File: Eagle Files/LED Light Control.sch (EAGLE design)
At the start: 9 parts, among them IC1 LM317MBSTT3

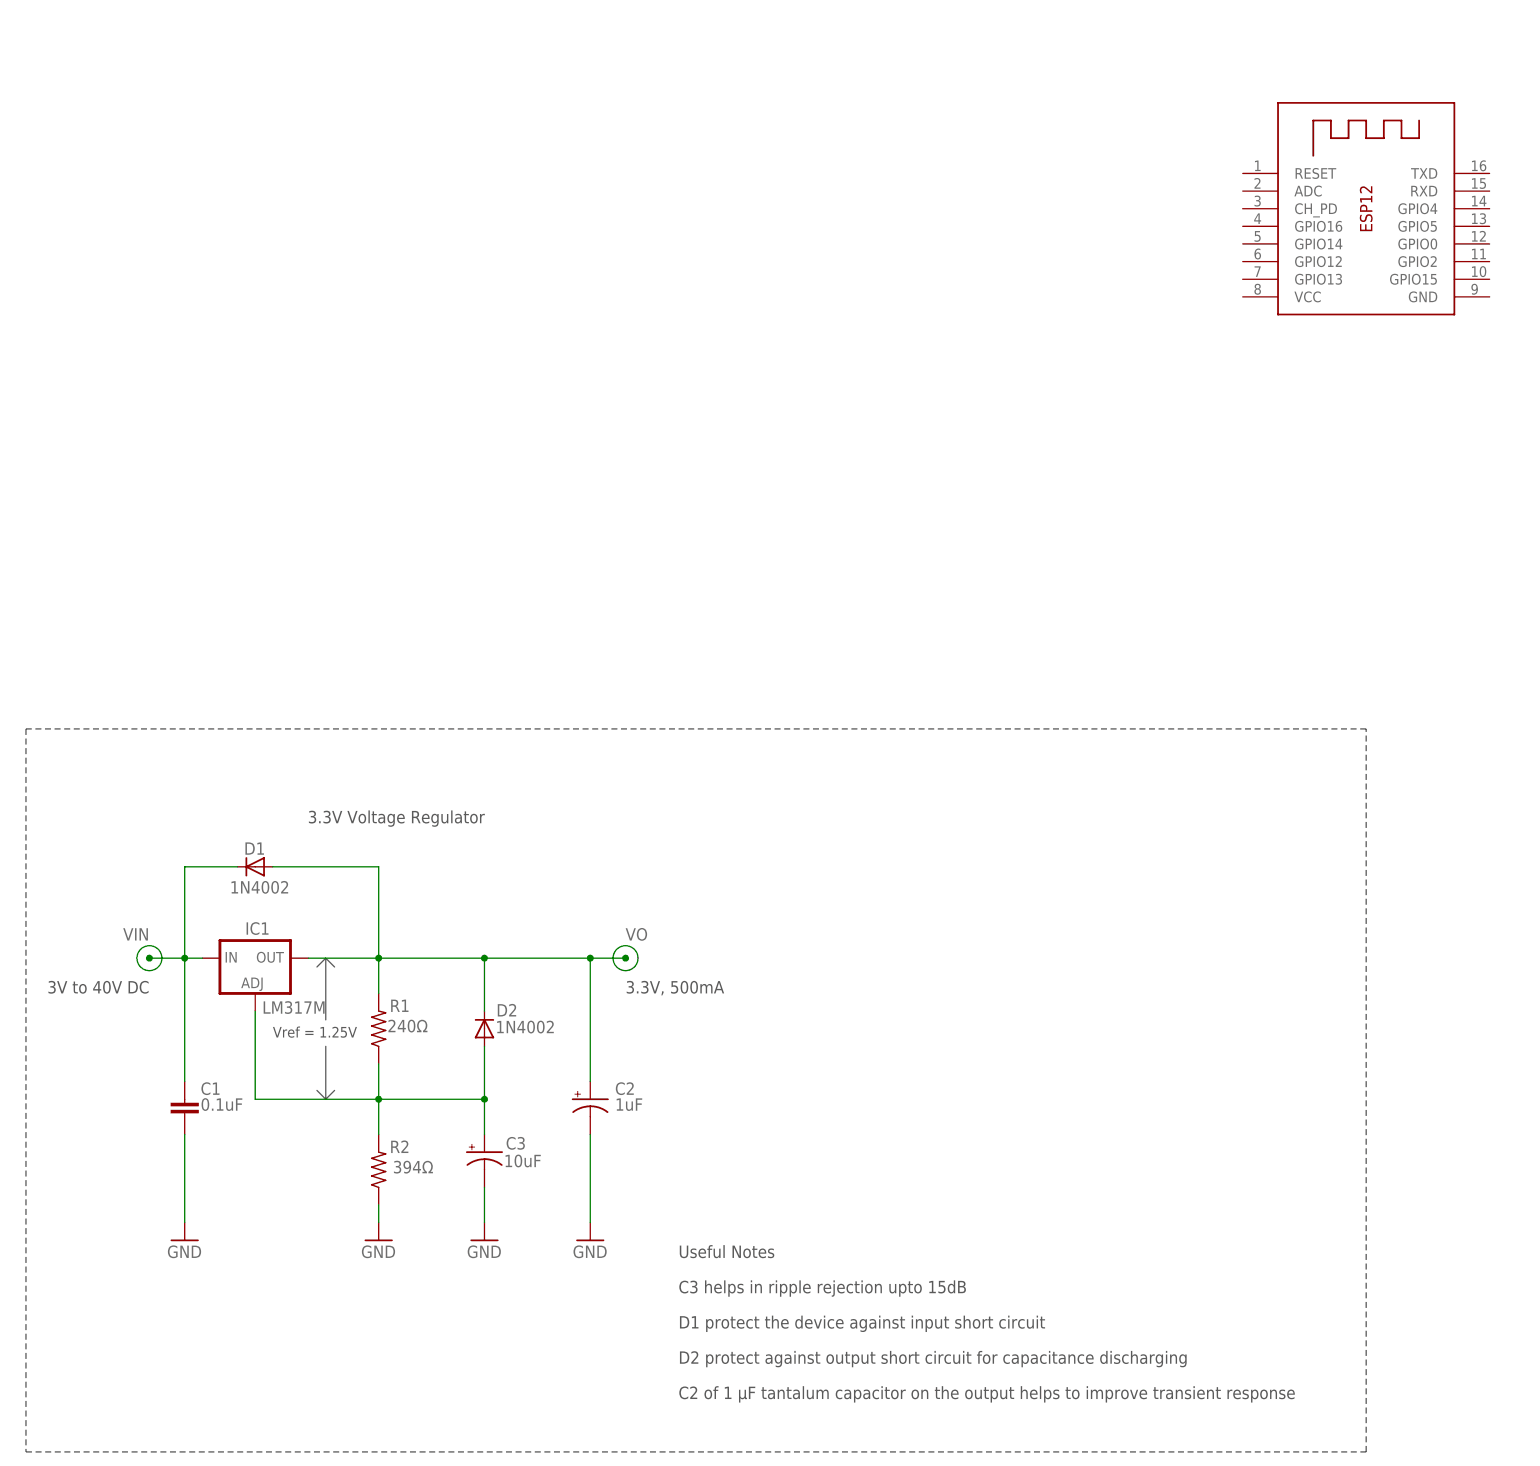
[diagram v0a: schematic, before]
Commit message: Added plans for the board
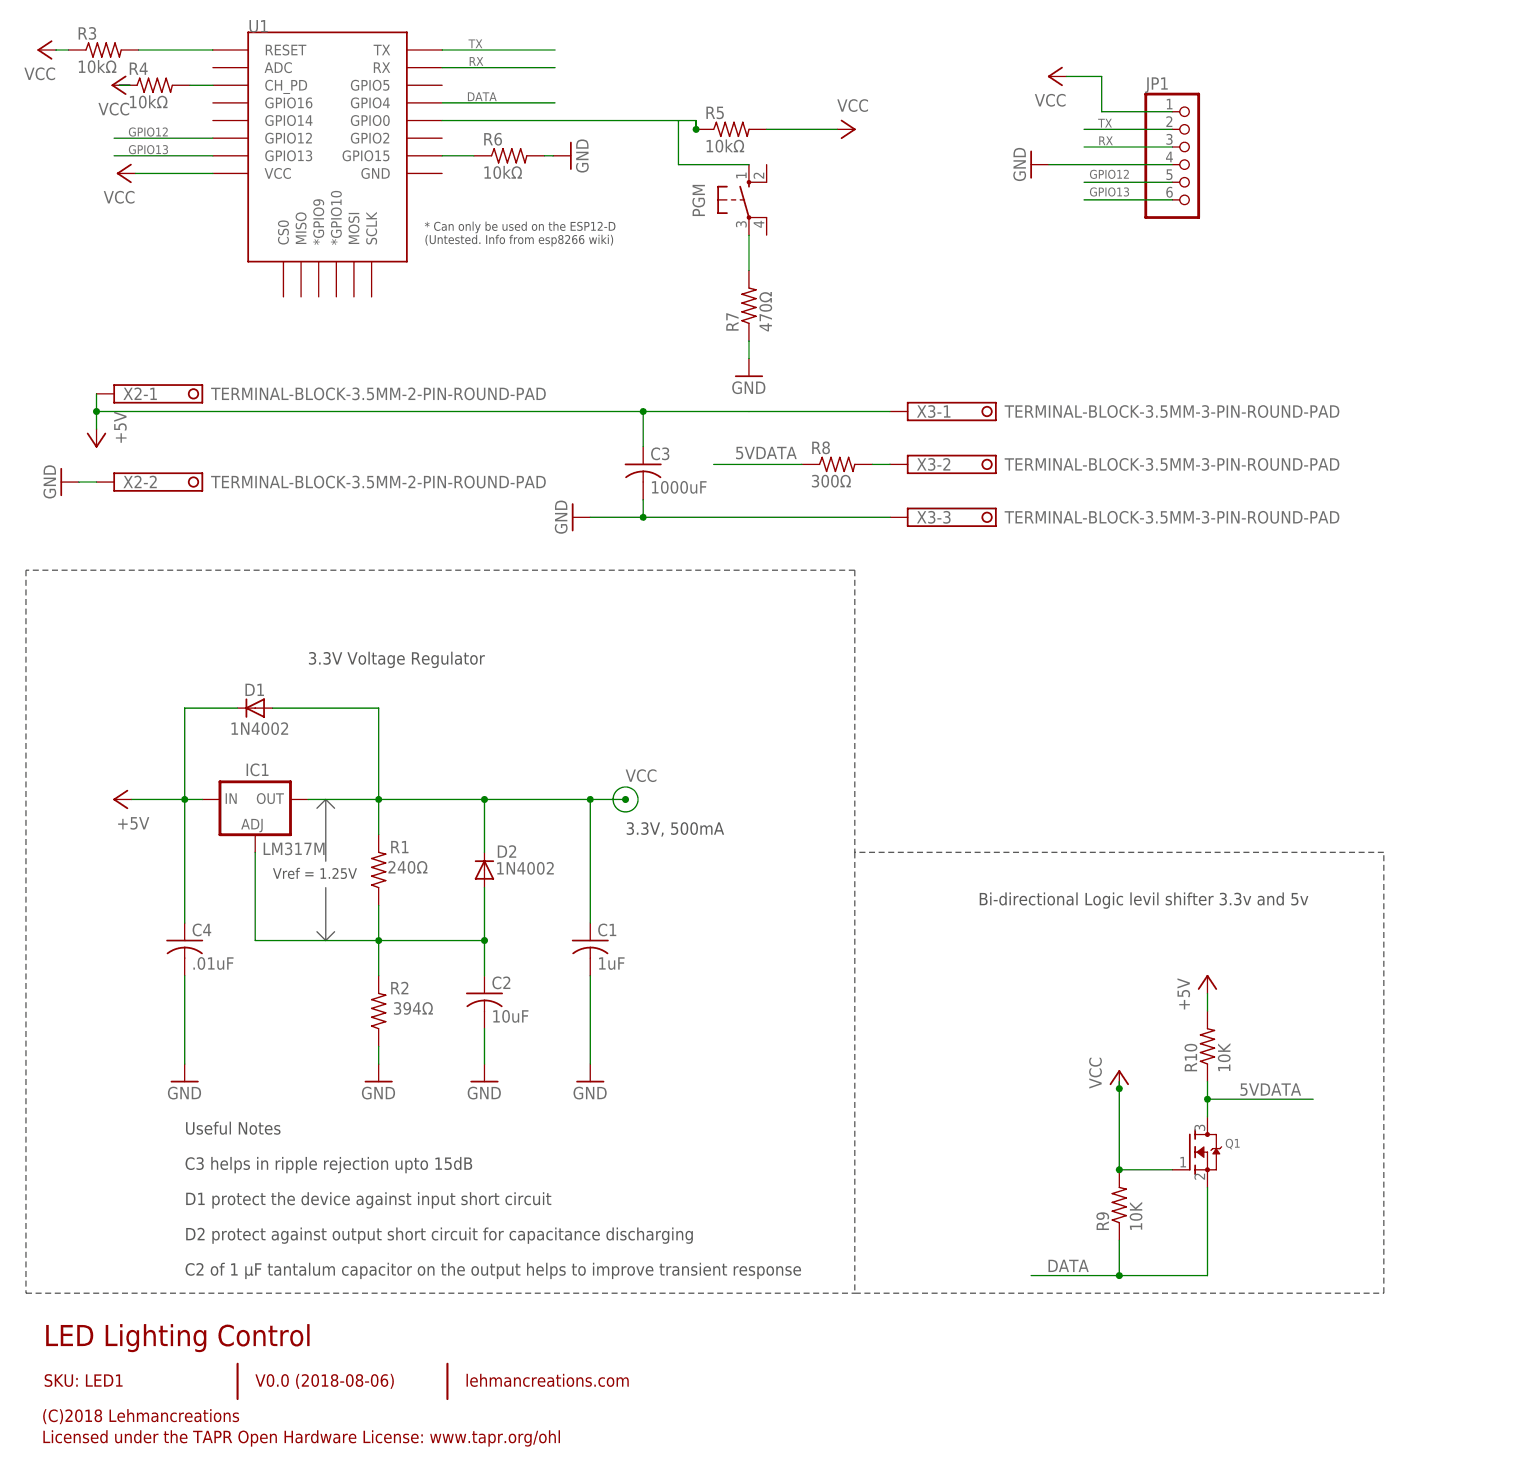
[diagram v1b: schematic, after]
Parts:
- removed X1: (no value), adafruit:ESP-12
- added C4: .01uF, adafruit:C-USC0805
- added JP1: (no value), adafruit:PINHD-1X6
- added PGM: (no value), switch-omron:10-XX
- added Q1: (no value), adafruit:MOSFET-NWAVE
- added R10, R9: 10K, adafruit:R-US_R0805
- added R3, R4, R5, R6: 10kΩ, adafruit:R-US_R0805
- added R7: 470Ω, adafruit:R-US_R0805
- added R8: 300Ω, adafruit:R-US_R0805
- added U1: (no value), esp8266modules:ESP12ESMD
- added X2: TERMINAL-BLOCK-3.5MM-2-PIN-ROUND-PAD, Rembrandt Electronics - Terminal Block 3-5mm v1-0:TERMINAL-BLOCK-3.5MM-2-PIN-ROUND-PAD
- added X3: TERMINAL-BLOCK-3.5MM-3-PIN-ROUND-PAD, Rembrandt Electronics - Terminal Block 3-5mm v1-0:TERMINAL-BLOCK-3.5MM-3-PIN-ROUND-PAD
- C1: value 0.1uF -> 1uF; device rcl:C-EU075-052X106 -> adafruit:C-USC0805
- C2: value 1uF -> 10uF; device resistor:CPOL-US085CS-1AR -> adafruit:C-USC0805
- C3: value 10uF -> 1000uF; device resistor:CPOL-US085CS-1AR -> adafruit:C-USC0805
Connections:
- removed net VIN: C1.1, D1.C, IC1.IN
- removed net VO: C2.+, D1.A, D2.C, IC1.OUT, R1.2
- new net +5V: C3.1, C4.1, D1.C, IC1.IN, R10.2, X2-1.K, X3-1.K
- new net 5VDATA: Q1.D, R10.1, R8.1
- new net DATA: Q1.S, R9.1, U1.GPIO4
- new net GPIO12: JP1.5, U1.GPIO12
- new net GPIO13: JP1.6, U1.GPIO13
- new net N$2: R3.2, U1.RESET
- new net N$3: R4.2, U1.CH_PD
- new net N$5: R6.1, U1.GPIO15
- new net N$6: PGM.P, R7.2
- new net N$7: R8.2, X3-2.K
- new net N$9: PGM.S, R5.1, U1.GPIO0
- new net RX: JP1.3, U1.RX
- new net TX: JP1.2, U1.TX
- new net VCC: C1.1, D1.A, D2.C, IC1.OUT, JP1.1, Q1.G, R1.2, R3.1, R4.1, R5.2, R9.2, U1.VCC
- net GND: now also C2.2, C3.2, C4.2, JP1.4, R6.2, R7.1, X2-2.K, X3-3.K; no longer C2.-, C3.-
- net N$1: now also C2.1; no longer C3.+
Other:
- note added: "(C)2018 Lehmancreations"
- note added: "Bi-directional Logic levil shifter 3.3v and 5v"
- note added: "LED Lighting Control"
- note added: "Licensed under the TAPR Open Hardware License: www.tapr.org/ohl"
- note added: "SKU: LED1"
- note added: "V0.0 (2018-08-06)"
- note added: "lehmancreations.com"
- note removed: "3V to 40V DC"
- moved on the sheet: C1, D1, D2, IC1, R1, R2

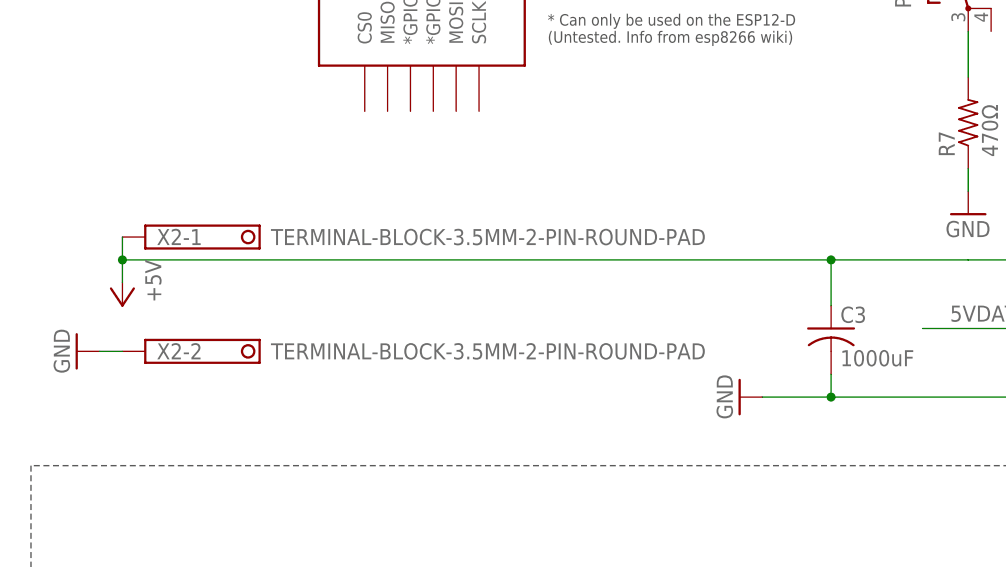
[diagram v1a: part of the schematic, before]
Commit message: Changes
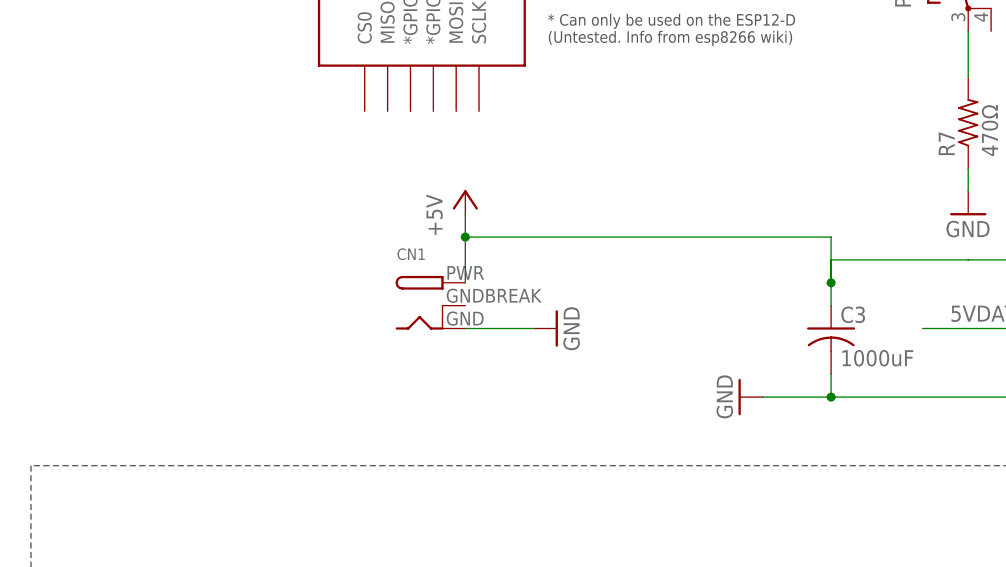
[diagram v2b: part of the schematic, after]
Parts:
- removed X2: TERMINAL-BLOCK-3.5MM-2-PIN-ROUND-PAD, Rembrandt Electronics - Terminal Block 3-5mm v1-0:TERMINAL-BLOCK-3.5MM-2-PIN-ROUND-PAD
- added CN1: (no value), adafruit:DCBARRELPTH
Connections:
- net +5V: now also CN1.PWR; no longer X2-1.K
- net GND: now also CN1.GND; no longer X2-2.K
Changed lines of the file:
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@@
 <part name="C1" library="adafruit" deviceset="C-US" device="C0805" value="1uF"/>
 <part name="C2" library="adafruit" deviceset="C-US" device="C0805" value="10uF"/>
-<part name="X2" library="Rembrandt Electronics - Terminal Block 3-5mm v1-0" deviceset="TERMINAL-BLOCK-3.5MM-2-PIN" device="-ROUND-PAD"/>
 <part name="SUPPLY7" library="supply1" library_urn="urn:adsk.eagle:library:371" deviceset="GND" device=""/>
 <part name="X3" library="Rembrandt Electronics - Terminal Block 3-5mm v1-0" deviceset="TERMINAL-BLOCK-3.5MM-3-PIN" device="-ROUND-PAD"/>
@@
 <part name="P+9" library="supply1" library_urn="urn:adsk.eagle:library:371" deviceset="+5V" device=""/>
 <part name="U1" library="esp8266modules" deviceset="ESP12E" device="SMD"/>
+<part name="CN1" library="adafruit" deviceset="DCBARREL" device="PTH"/>
 </parts>
 <sheets>
@@
 <instance part="C1" gate="G$1" x="81.28" y="73.66"/>
 <instance part="C2" gate="G$1" x="66.04" y="66.04"/>
-<instance part="X2" gate="-1" x="12.7" y="152.4"/>
-<instance part="X2" gate="-2" x="12.7" y="139.7"/>
-<instance part="SUPPLY7" gate="1" x="5.08" y="139.7" rot="R270"/>
+<instance part="SUPPLY7" gate="1" x="58.42" y="142.24" rot="R90"/>
 <instance part="X3" gate="-1" x="127" y="149.86"/>
 <instance part="X3" gate="-2" x="127" y="142.24"/>
@@
 <instance part="R10" gate="G$1" x="170.18" y="58.42" rot="R90"/>
 <instance part="P+6" gate="VCC" x="157.48" y="54.864"/>
-<instance part="P+7" gate="1" x="10.16" y="144.78" rot="R180"/>
+<instance part="P+7" gate="1" x="48.26" y="157.48"/>
 <instance part="P+8" gate="1" x="12.7" y="93.98" rot="R90"/>
 <instance part="P+9" gate="1" x="170.18" y="68.58"/>
 <instance part="U1" gate="G$1" x="44.704" y="194.31"/>
+<instance part="CN1" gate="G$1" x="45.72" y="144.78"/>
 </instances>
 <busses>
@@
 <pinref part="SUPPLY5" gate="1" pin="GND"/>
 <wire x1="74.676" y1="186.69" x2="75.946" y2="186.69" width="0.1524" layer="91"/>
-</segment>
-<segment>
-<pinref part="SUPPLY7" gate="1" pin="GND"/>
-<pinref part="X2" gate="-2" pin="K"/>
-<wire x1="7.62" y1="139.7" x2="10.16" y2="139.7" width="0.1524" layer="91"/>
 </segment>
 <segment>
@@
 <pinref part="SUPPLY9" gate="1" pin="GND"/>
 <wire x1="165.1" y1="185.42" x2="147.32" y2="185.42" width="0.1524" layer="91"/>
+</segment>
+<segment>
+<pinref part="CN1" gate="G$1" pin="GND"/>
+<pinref part="SUPPLY7" gate="1" pin="GND"/>
+<wire x1="48.26" y1="142.24" x2="55.88" y2="142.24" width="0.1524" layer="91"/>
 </segment>
 </net>
@@
 <net name="+5V" class="0">
 <segment>
-<pinref part="X2" gate="-1" pin="K"/>
-<wire x1="10.16" y1="152.4" x2="10.16" y2="149.86" width="0.1524" layer="91"/>
-<pinref part="X3" gate="-1" pin="K"/>
-<wire x1="124.46" y1="149.86" x2="104.14" y2="149.86" width="0.1524" layer="91"/>
-<wire x1="104.14" y1="149.86" x2="88.9" y2="149.86" width="0.1524" layer="91"/>
-<wire x1="88.9" y1="149.86" x2="10.16" y2="149.86" width="0.1524" layer="91"/>
-<wire x1="10.16" y1="147.32" x2="10.16" y2="149.86" width="0.1524" layer="91"/>
-<junction x="10.16" y="149.86"/>
-<pinref part="P+7" gate="1" pin="+5V"/>
-<pinref part="C3" gate="G$1" pin="1"/>
-<wire x1="88.9" y1="144.78" x2="88.9" y2="149.86" width="0.1524" layer="91"/>
-<junction x="88.9" y="149.86"/>
-</segment>
-<segment>
 <pinref part="IC1" gate="G$1" pin="IN"/>
 <wire x1="25.4" y1="93.98" x2="22.86" y2="93.98" width="0.1524" layer="91"/>
@@
 <pinref part="P+9" gate="1" pin="+5V"/>
 </segment>
-</net>
+<segment>
+<pinref part="CN1" gate="G$1" pin="PWR"/>
+<pinref part="P+7" gate="1" pin="+5V"/>
+<wire x1="48.26" y1="147.32" x2="48.26" y2="152.4" width="0.1524" layer="91"/>
+<pinref part="X3" gate="-1" pin="K"/>
+<wire x1="48.26" y1="152.4" x2="48.26" y2="154.94" width="0.1524" layer="91"/>
+<wire x1="124.46" y1="149.86" x2="104.14" y2="149.86" width="0.1524" layer="91"/>
+<wire x1="104.14" y1="149.86" x2="88.9" y2="149.86" width="0.1524" layer="91"/>
+<pinref part="C3" gate="G$1" pin="1"/>
+<wire x1="88.9" y1="144.78" x2="88.9" y2="147.32" width="0.1524" layer="91"/>
+<wire x1="88.9" y1="147.32" x2="88.9" y2="149.86" width="0.1524" layer="91"/>
+<wire x1="48.26" y1="152.4" x2="88.9" y2="152.4" width="0.1524" layer="91"/>
+<wire x1="88.9" y1="152.4" x2="88.9" y2="147.32" width="0.1524" layer="91"/>
+<junction x="48.26" y="152.4"/>
+<junction x="88.9" y="147.32"/>
+</segment>
+</net>
